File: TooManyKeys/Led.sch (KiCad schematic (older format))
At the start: 2 parts

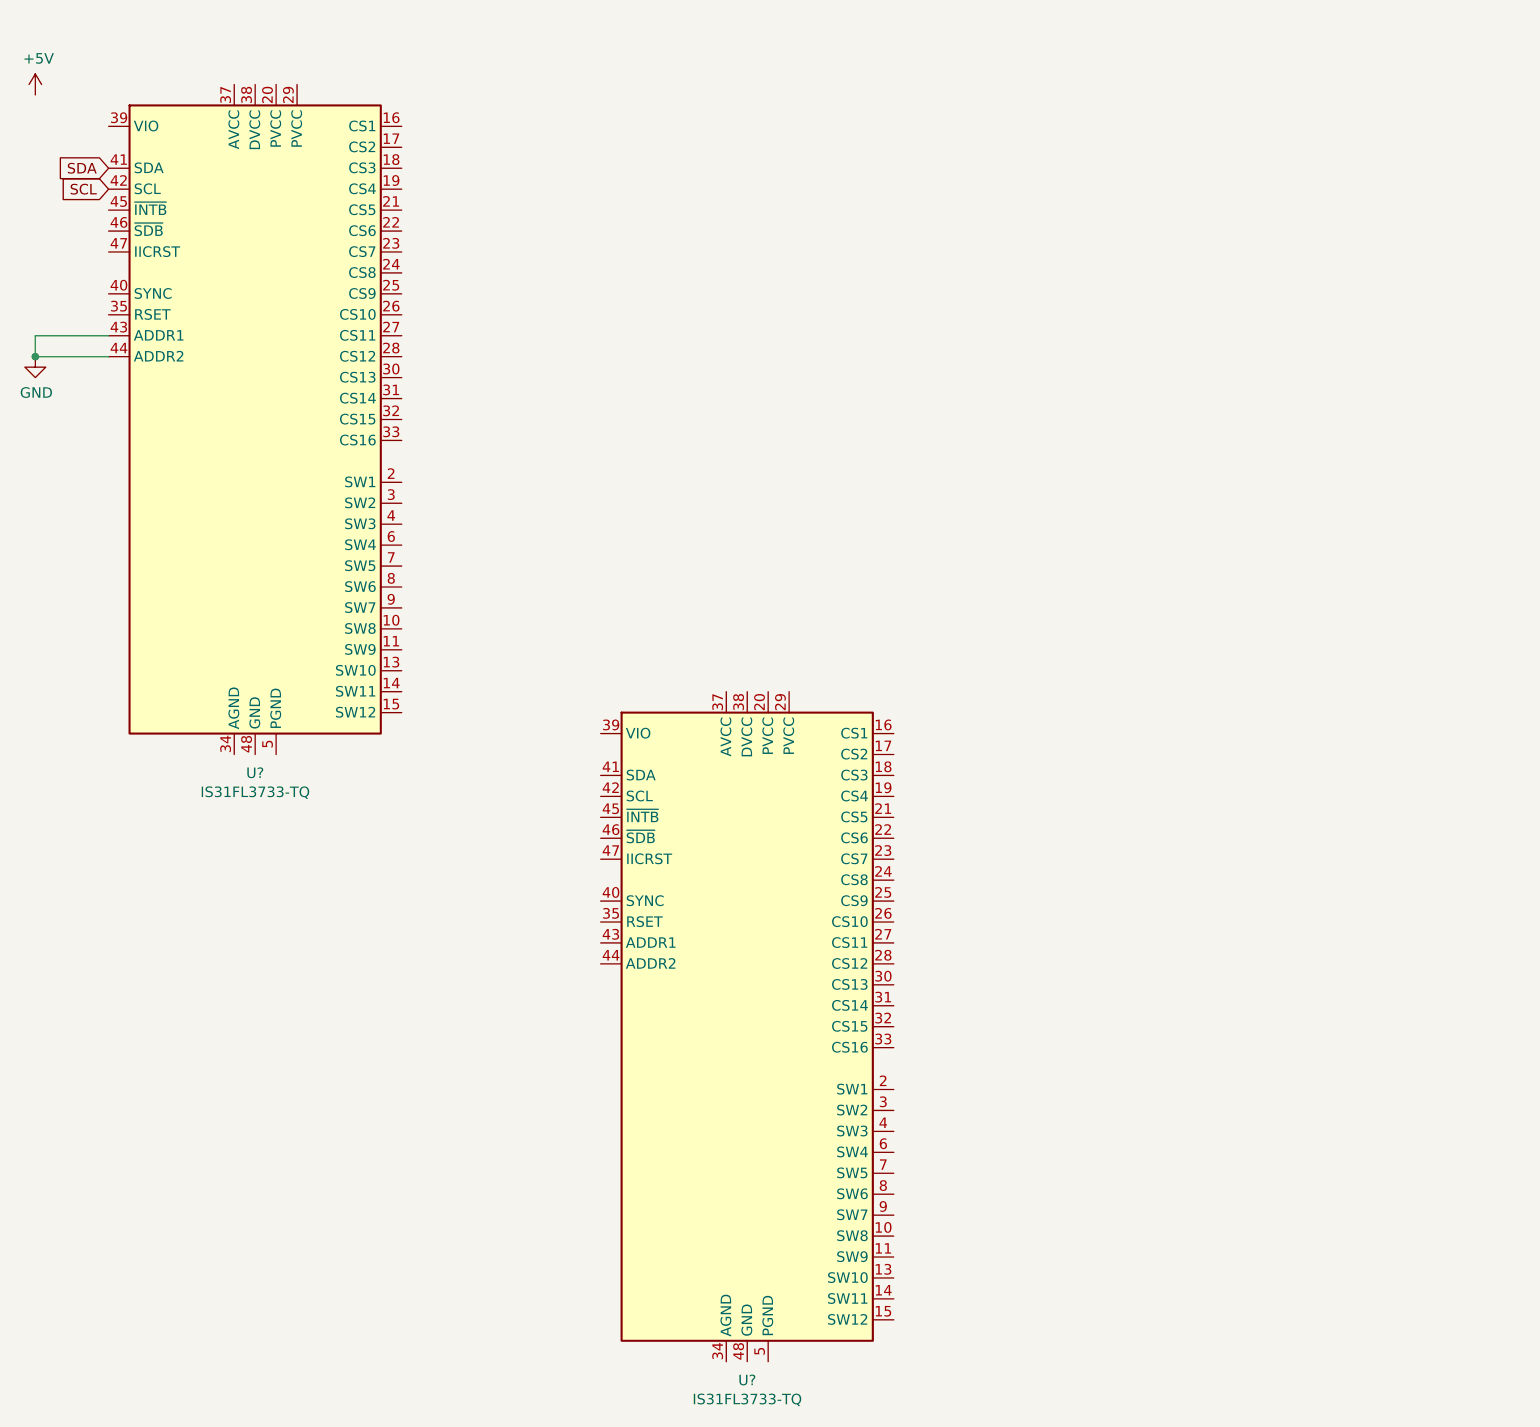
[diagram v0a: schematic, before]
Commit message: led work
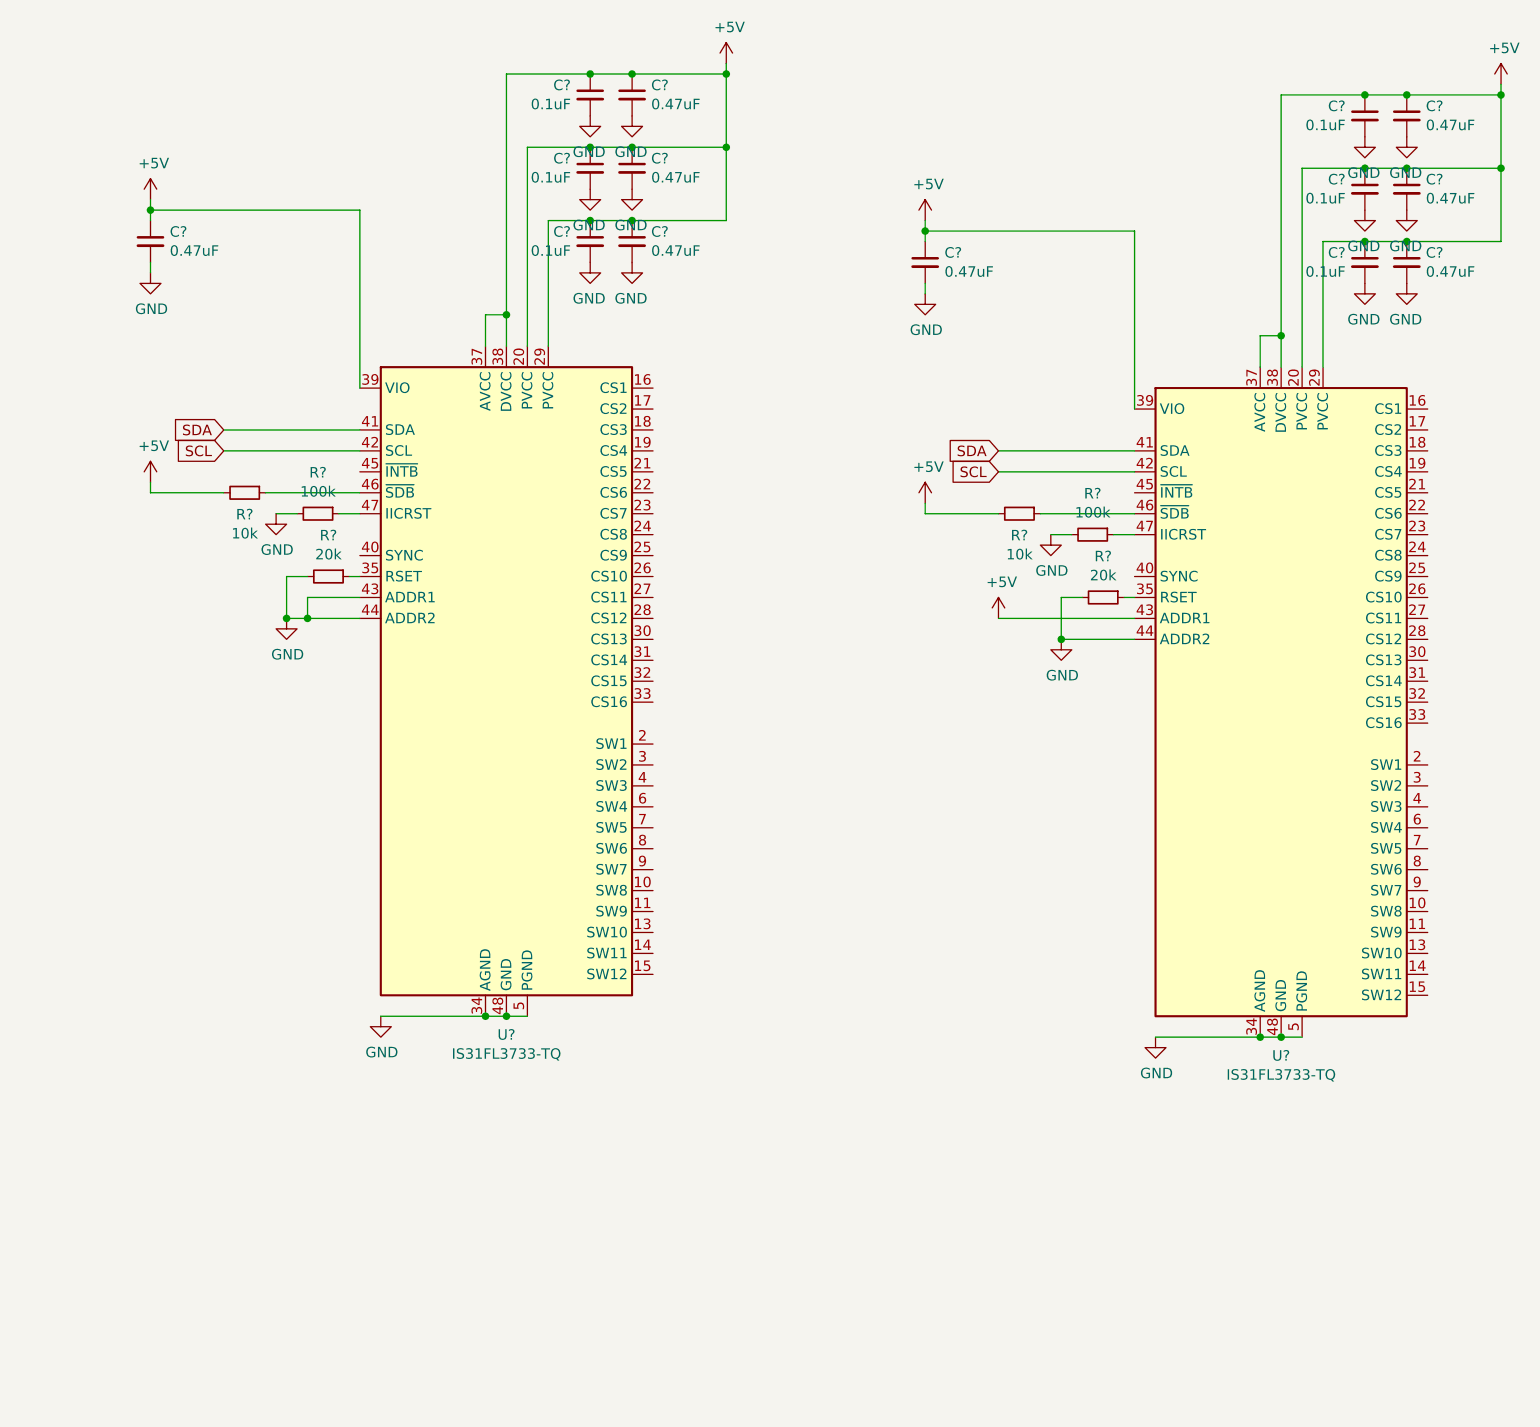
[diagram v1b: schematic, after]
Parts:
- removed U?: IS31FL3733-TQ, Package_QFP:TQFP-48-1EP_7x7mm_P0.5mm_EP5x5mm, symbol Driver_LED:IS31FL3733-TQ
- added C? (x8): 0.47uF, symbol Device:C_Small
- added C? (x6): 0.1uF, symbol Device:C_Small
- added R? (x2): 100k, symbol Device:R_Small
- added R? (x2): 20k, symbol Device:R_Small
- added R? (x2): 10k, symbol Device:R_Small
- added U?: IS31FL3733-TQ, Package_QFP:TQFP-48-1EP_7x7mm_P0.5mm_EP5x5mm, symbol Driver_LED:IS31FL3733-TQ
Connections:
- net +5V: now also U?.20 (PVCC), U?.29 (PVCC), U?.37 (AVCC), U?.38 (DVCC), U?.39 (VIO), C?.1, C?.1, C?.1, C?.1, C?.1, C?.1, C?.1, C?.1, C?.1, C?.1, C?.1, C?.1, C?.1, C?.1, R?.2, R?.2, U?.20 (PVCC), U?.29 (PVCC), U?.37 (AVCC), U?.38 (DVCC), U?.39 (VIO), U?.43 (ADDR1)
- net GND: now also U?.12 (PGND), U?.34 (AGND), U?.48 (GND), U?.49 (GND), U?.5 (PGND), C?.2, C?.2, C?.2, C?.2, C?.2, C?.2, C?.2, C?.2, C?.2, C?.2, C?.2, C?.2, C?.2, C?.2, R?.2, R?.2, R?.2, R?.2, U?.12 (PGND), U?.34 (AGND), U?.44 (ADDR2), U?.48 (GND), U?.49 (GND), U?.5 (PGND)
- net SCL: now also U?.42 (SCL)
- net SDA: now also U?.41 (SDA)
- net at U?.35 (RSET): now also R?.1
- net at U?.46 (~SDB): now also R?.1
- net at U?.47 (IICRST): now also R?.1
- new net: R?.1, U?.35 (RSET)
- new net: R?.1, U?.46 (~SDB)
- new net: R?.1, U?.47 (IICRST)
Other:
- moved on the sheet: U?

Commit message: Adding led matrix
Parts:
- added LED? (x64): XZMDKCBDDG45S-9, XZMDKCBDDG45S9, symbol SamacSys_Parts:XZMDKCBDDG45S-9
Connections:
- new net CS1: LED?.2 (COMMON_ANODE), LED?.2 (COMMON_ANODE), LED?.2 (COMMON_ANODE), LED?.2 (COMMON_ANODE)
- new net CS10: LED?.2 (COMMON_ANODE), LED?.2 (COMMON_ANODE), LED?.2 (COMMON_ANODE), LED?.2 (COMMON_ANODE)
- new net CS11: LED?.2 (COMMON_ANODE), LED?.2 (COMMON_ANODE), LED?.2 (COMMON_ANODE), LED?.2 (COMMON_ANODE)
- new net CS12: LED?.2 (COMMON_ANODE), LED?.2 (COMMON_ANODE), LED?.2 (COMMON_ANODE), LED?.2 (COMMON_ANODE)
- new net CS13: LED?.2 (COMMON_ANODE), LED?.2 (COMMON_ANODE), LED?.2 (COMMON_ANODE), LED?.2 (COMMON_ANODE)
- new net CS14: LED?.2 (COMMON_ANODE), LED?.2 (COMMON_ANODE), LED?.2 (COMMON_ANODE), LED?.2 (COMMON_ANODE)
- new net CS15: LED?.2 (COMMON_ANODE), LED?.2 (COMMON_ANODE), LED?.2 (COMMON_ANODE), LED?.2 (COMMON_ANODE)
- new net CS16: LED?.2 (COMMON_ANODE), LED?.2 (COMMON_ANODE), LED?.2 (COMMON_ANODE), LED?.2 (COMMON_ANODE)
- new net CS2: LED?.2 (COMMON_ANODE), LED?.2 (COMMON_ANODE), LED?.2 (COMMON_ANODE), LED?.2 (COMMON_ANODE)
- new net CS3: LED?.2 (COMMON_ANODE), LED?.2 (COMMON_ANODE), LED?.2 (COMMON_ANODE), LED?.2 (COMMON_ANODE)
- new net CS4: LED?.2 (COMMON_ANODE), LED?.2 (COMMON_ANODE), LED?.2 (COMMON_ANODE), LED?.2 (COMMON_ANODE)
- new net CS5: LED?.2 (COMMON_ANODE), LED?.2 (COMMON_ANODE), LED?.2 (COMMON_ANODE), LED?.2 (COMMON_ANODE)
- new net CS6: LED?.2 (COMMON_ANODE), LED?.2 (COMMON_ANODE), LED?.2 (COMMON_ANODE), LED?.2 (COMMON_ANODE)
- new net CS7: LED?.2 (COMMON_ANODE), LED?.2 (COMMON_ANODE), LED?.2 (COMMON_ANODE), LED?.2 (COMMON_ANODE)
- new net CS8: LED?.2 (COMMON_ANODE), LED?.2 (COMMON_ANODE), LED?.2 (COMMON_ANODE), LED?.2 (COMMON_ANODE)
- new net CS9: LED?.2 (COMMON_ANODE), LED?.2 (COMMON_ANODE), LED?.2 (COMMON_ANODE), LED?.2 (COMMON_ANODE)
- new net SW1: LED?.4 (CATHODE_GREEN), LED?.4 (CATHODE_GREEN), LED?.4 (CATHODE_GREEN), LED?.4 (CATHODE_GREEN), LED?.4 (CATHODE_GREEN), LED?.4 (CATHODE_GREEN), LED?.4 (CATHODE_GREEN), LED?.4 (CATHODE_GREEN), LED?.4 (CATHODE_GREEN), LED?.4 (CATHODE_GREEN), LED?.4 (CATHODE_GREEN), LED?.4 (CATHODE_GREEN), LED?.4 (CATHODE_GREEN), LED?.4 (CATHODE_GREEN), LED?.4 (CATHODE_GREEN), LED?.4 (CATHODE_GREEN)
- new net SW10: LED?.4 (CATHODE_GREEN), LED?.4 (CATHODE_GREEN), LED?.4 (CATHODE_GREEN), LED?.4 (CATHODE_GREEN), LED?.4 (CATHODE_GREEN), LED?.4 (CATHODE_GREEN), LED?.4 (CATHODE_GREEN), LED?.4 (CATHODE_GREEN), LED?.4 (CATHODE_GREEN), LED?.4 (CATHODE_GREEN), LED?.4 (CATHODE_GREEN), LED?.4 (CATHODE_GREEN), LED?.4 (CATHODE_GREEN), LED?.4 (CATHODE_GREEN), LED?.4 (CATHODE_GREEN), LED?.4 (CATHODE_GREEN)
- new net SW11: LED?.1 (CATHODE_RED), LED?.1 (CATHODE_RED), LED?.1 (CATHODE_RED), LED?.1 (CATHODE_RED), LED?.1 (CATHODE_RED), LED?.1 (CATHODE_RED), LED?.1 (CATHODE_RED), LED?.1 (CATHODE_RED), LED?.1 (CATHODE_RED), LED?.1 (CATHODE_RED), LED?.1 (CATHODE_RED), LED?.1 (CATHODE_RED), LED?.1 (CATHODE_RED), LED?.1 (CATHODE_RED), LED?.1 (CATHODE_RED), LED?.1 (CATHODE_RED)
- new net SW12: LED?.3 (CATHODE_BLUE), LED?.3 (CATHODE_BLUE), LED?.3 (CATHODE_BLUE), LED?.3 (CATHODE_BLUE), LED?.3 (CATHODE_BLUE), LED?.3 (CATHODE_BLUE), LED?.3 (CATHODE_BLUE), LED?.3 (CATHODE_BLUE), LED?.3 (CATHODE_BLUE), LED?.3 (CATHODE_BLUE), LED?.3 (CATHODE_BLUE), LED?.3 (CATHODE_BLUE), LED?.3 (CATHODE_BLUE), LED?.3 (CATHODE_BLUE), LED?.3 (CATHODE_BLUE), LED?.3 (CATHODE_BLUE)
- new net SW2: LED?.1 (CATHODE_RED), LED?.1 (CATHODE_RED), LED?.1 (CATHODE_RED), LED?.1 (CATHODE_RED), LED?.1 (CATHODE_RED), LED?.1 (CATHODE_RED), LED?.1 (CATHODE_RED), LED?.1 (CATHODE_RED), LED?.1 (CATHODE_RED), LED?.1 (CATHODE_RED), LED?.1 (CATHODE_RED), LED?.1 (CATHODE_RED), LED?.1 (CATHODE_RED), LED?.1 (CATHODE_RED), LED?.1 (CATHODE_RED), LED?.1 (CATHODE_RED)
- new net SW3: LED?.3 (CATHODE_BLUE), LED?.3 (CATHODE_BLUE), LED?.3 (CATHODE_BLUE), LED?.3 (CATHODE_BLUE), LED?.3 (CATHODE_BLUE), LED?.3 (CATHODE_BLUE), LED?.3 (CATHODE_BLUE), LED?.3 (CATHODE_BLUE), LED?.3 (CATHODE_BLUE), LED?.3 (CATHODE_BLUE), LED?.3 (CATHODE_BLUE), LED?.3 (CATHODE_BLUE), LED?.3 (CATHODE_BLUE), LED?.3 (CATHODE_BLUE), LED?.3 (CATHODE_BLUE), LED?.3 (CATHODE_BLUE)
- new net SW4: LED?.4 (CATHODE_GREEN), LED?.4 (CATHODE_GREEN), LED?.4 (CATHODE_GREEN), LED?.4 (CATHODE_GREEN), LED?.4 (CATHODE_GREEN), LED?.4 (CATHODE_GREEN), LED?.4 (CATHODE_GREEN), LED?.4 (CATHODE_GREEN), LED?.4 (CATHODE_GREEN), LED?.4 (CATHODE_GREEN), LED?.4 (CATHODE_GREEN), LED?.4 (CATHODE_GREEN), LED?.4 (CATHODE_GREEN), LED?.4 (CATHODE_GREEN), LED?.4 (CATHODE_GREEN), LED?.4 (CATHODE_GREEN)
- new net SW5: LED?.1 (CATHODE_RED), LED?.1 (CATHODE_RED), LED?.1 (CATHODE_RED), LED?.1 (CATHODE_RED), LED?.1 (CATHODE_RED), LED?.1 (CATHODE_RED), LED?.1 (CATHODE_RED), LED?.1 (CATHODE_RED), LED?.1 (CATHODE_RED), LED?.1 (CATHODE_RED), LED?.1 (CATHODE_RED), LED?.1 (CATHODE_RED), LED?.1 (CATHODE_RED), LED?.1 (CATHODE_RED), LED?.1 (CATHODE_RED), LED?.1 (CATHODE_RED)
- new net SW6: LED?.3 (CATHODE_BLUE), LED?.3 (CATHODE_BLUE), LED?.3 (CATHODE_BLUE), LED?.3 (CATHODE_BLUE), LED?.3 (CATHODE_BLUE), LED?.3 (CATHODE_BLUE), LED?.3 (CATHODE_BLUE), LED?.3 (CATHODE_BLUE), LED?.3 (CATHODE_BLUE), LED?.3 (CATHODE_BLUE), LED?.3 (CATHODE_BLUE), LED?.3 (CATHODE_BLUE), LED?.3 (CATHODE_BLUE), LED?.3 (CATHODE_BLUE), LED?.3 (CATHODE_BLUE), LED?.3 (CATHODE_BLUE)
- new net SW7: LED?.4 (CATHODE_GREEN), LED?.4 (CATHODE_GREEN), LED?.4 (CATHODE_GREEN), LED?.4 (CATHODE_GREEN), LED?.4 (CATHODE_GREEN), LED?.4 (CATHODE_GREEN), LED?.4 (CATHODE_GREEN), LED?.4 (CATHODE_GREEN), LED?.4 (CATHODE_GREEN), LED?.4 (CATHODE_GREEN), LED?.4 (CATHODE_GREEN), LED?.4 (CATHODE_GREEN), LED?.4 (CATHODE_GREEN), LED?.4 (CATHODE_GREEN), LED?.4 (CATHODE_GREEN), LED?.4 (CATHODE_GREEN)
- new net SW8: LED?.1 (CATHODE_RED), LED?.1 (CATHODE_RED), LED?.1 (CATHODE_RED), LED?.1 (CATHODE_RED), LED?.1 (CATHODE_RED), LED?.1 (CATHODE_RED), LED?.1 (CATHODE_RED), LED?.1 (CATHODE_RED), LED?.1 (CATHODE_RED), LED?.1 (CATHODE_RED), LED?.1 (CATHODE_RED), LED?.1 (CATHODE_RED), LED?.1 (CATHODE_RED), LED?.1 (CATHODE_RED), LED?.1 (CATHODE_RED), LED?.1 (CATHODE_RED)
- new net SW9: LED?.3 (CATHODE_BLUE), LED?.3 (CATHODE_BLUE), LED?.3 (CATHODE_BLUE), LED?.3 (CATHODE_BLUE), LED?.3 (CATHODE_BLUE), LED?.3 (CATHODE_BLUE), LED?.3 (CATHODE_BLUE), LED?.3 (CATHODE_BLUE), LED?.3 (CATHODE_BLUE), LED?.3 (CATHODE_BLUE), LED?.3 (CATHODE_BLUE), LED?.3 (CATHODE_BLUE), LED?.3 (CATHODE_BLUE), LED?.3 (CATHODE_BLUE), LED?.3 (CATHODE_BLUE), LED?.3 (CATHODE_BLUE)
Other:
- moved on the sheet: C?, R?, U?

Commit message: V1 Schematics
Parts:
- removed C? (x8): 0.47uF, symbol Device:C_Small
- removed C? (x6): 0.1uF, symbol Device:C_Small
- removed R? (x2): 100k, symbol Device:R_Small
- removed R? (x2): 20k, symbol Device:R_Small
- removed R? (x2): 10k, symbol Device:R_Small
- removed U? (x2): IS31FL3733-TQ, Package_QFP:TQFP-48-1EP_7x7mm_P0.5mm_EP5x5mm, symbol Driver_LED:IS31FL3733-TQ
- added LED? (x47): XZMDKCBDDG45S-9, XZMDKCBDDG45S9, symbol SamacSys_Parts:XZMDKCBDDG45S-9
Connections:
- new net CS17: LED?.2 (COMMON_ANODE), LED?.2 (COMMON_ANODE), LED?.2 (COMMON_ANODE), LED?.2 (COMMON_ANODE)
- new net CS18: LED?.2 (COMMON_ANODE), LED?.2 (COMMON_ANODE), LED?.2 (COMMON_ANODE), LED?.2 (COMMON_ANODE)
- new net CS19: LED?.2 (COMMON_ANODE), LED?.2 (COMMON_ANODE), LED?.2 (COMMON_ANODE), LED?.2 (COMMON_ANODE)
- new net CS20: LED?.2 (COMMON_ANODE), LED?.2 (COMMON_ANODE), LED?.2 (COMMON_ANODE), LED?.2 (COMMON_ANODE)
- new net CS21: LED?.2 (COMMON_ANODE), LED?.2 (COMMON_ANODE), LED?.2 (COMMON_ANODE), LED?.2 (COMMON_ANODE)
- new net CS22: LED?.2 (COMMON_ANODE), LED?.2 (COMMON_ANODE), LED?.2 (COMMON_ANODE), LED?.2 (COMMON_ANODE)
- new net CS23: LED?.2 (COMMON_ANODE), LED?.2 (COMMON_ANODE), LED?.2 (COMMON_ANODE), LED?.2 (COMMON_ANODE)
- new net CS24: LED?.2 (COMMON_ANODE), LED?.2 (COMMON_ANODE), LED?.2 (COMMON_ANODE), LED?.2 (COMMON_ANODE)
- new net CS25: LED?.2 (COMMON_ANODE), LED?.2 (COMMON_ANODE), LED?.2 (COMMON_ANODE), LED?.2 (COMMON_ANODE)
- new net CS26: LED?.2 (COMMON_ANODE), LED?.2 (COMMON_ANODE), LED?.2 (COMMON_ANODE), LED?.2 (COMMON_ANODE)
- new net CS27: LED?.2 (COMMON_ANODE), LED?.2 (COMMON_ANODE), LED?.2 (COMMON_ANODE), LED?.2 (COMMON_ANODE)
- new net CS28: LED?.2 (COMMON_ANODE), LED?.2 (COMMON_ANODE), LED?.2 (COMMON_ANODE)
- new net SW13: LED?.4 (CATHODE_GREEN), LED?.4 (CATHODE_GREEN), LED?.4 (CATHODE_GREEN), LED?.4 (CATHODE_GREEN), LED?.4 (CATHODE_GREEN), LED?.4 (CATHODE_GREEN), LED?.4 (CATHODE_GREEN), LED?.4 (CATHODE_GREEN), LED?.4 (CATHODE_GREEN), LED?.4 (CATHODE_GREEN), LED?.4 (CATHODE_GREEN), LED?.4 (CATHODE_GREEN)
- new net SW14: LED?.1 (CATHODE_RED), LED?.1 (CATHODE_RED), LED?.1 (CATHODE_RED), LED?.1 (CATHODE_RED), LED?.1 (CATHODE_RED), LED?.1 (CATHODE_RED), LED?.1 (CATHODE_RED), LED?.1 (CATHODE_RED), LED?.1 (CATHODE_RED), LED?.1 (CATHODE_RED), LED?.1 (CATHODE_RED), LED?.1 (CATHODE_RED)
- new net SW15: LED?.3 (CATHODE_BLUE), LED?.3 (CATHODE_BLUE), LED?.3 (CATHODE_BLUE), LED?.3 (CATHODE_BLUE), LED?.3 (CATHODE_BLUE), LED?.3 (CATHODE_BLUE), LED?.3 (CATHODE_BLUE), LED?.3 (CATHODE_BLUE), LED?.3 (CATHODE_BLUE), LED?.3 (CATHODE_BLUE), LED?.3 (CATHODE_BLUE), LED?.3 (CATHODE_BLUE)
- new net SW16: LED?.4 (CATHODE_GREEN), LED?.4 (CATHODE_GREEN), LED?.4 (CATHODE_GREEN), LED?.4 (CATHODE_GREEN), LED?.4 (CATHODE_GREEN), LED?.4 (CATHODE_GREEN), LED?.4 (CATHODE_GREEN), LED?.4 (CATHODE_GREEN), LED?.4 (CATHODE_GREEN), LED?.4 (CATHODE_GREEN), LED?.4 (CATHODE_GREEN), LED?.4 (CATHODE_GREEN)
- new net SW17: LED?.1 (CATHODE_RED), LED?.1 (CATHODE_RED), LED?.1 (CATHODE_RED), LED?.1 (CATHODE_RED), LED?.1 (CATHODE_RED), LED?.1 (CATHODE_RED), LED?.1 (CATHODE_RED), LED?.1 (CATHODE_RED), LED?.1 (CATHODE_RED), LED?.1 (CATHODE_RED), LED?.1 (CATHODE_RED), LED?.1 (CATHODE_RED)
- new net SW18: LED?.3 (CATHODE_BLUE), LED?.3 (CATHODE_BLUE), LED?.3 (CATHODE_BLUE), LED?.3 (CATHODE_BLUE), LED?.3 (CATHODE_BLUE), LED?.3 (CATHODE_BLUE), LED?.3 (CATHODE_BLUE), LED?.3 (CATHODE_BLUE), LED?.3 (CATHODE_BLUE), LED?.3 (CATHODE_BLUE), LED?.3 (CATHODE_BLUE), LED?.3 (CATHODE_BLUE)
- new net SW19: LED?.4 (CATHODE_GREEN), LED?.4 (CATHODE_GREEN), LED?.4 (CATHODE_GREEN), LED?.4 (CATHODE_GREEN), LED?.4 (CATHODE_GREEN), LED?.4 (CATHODE_GREEN), LED?.4 (CATHODE_GREEN), LED?.4 (CATHODE_GREEN), LED?.4 (CATHODE_GREEN), LED?.4 (CATHODE_GREEN), LED?.4 (CATHODE_GREEN), LED?.4 (CATHODE_GREEN)
- new net SW20: LED?.1 (CATHODE_RED), LED?.1 (CATHODE_RED), LED?.1 (CATHODE_RED), LED?.1 (CATHODE_RED), LED?.1 (CATHODE_RED), LED?.1 (CATHODE_RED), LED?.1 (CATHODE_RED), LED?.1 (CATHODE_RED), LED?.1 (CATHODE_RED), LED?.1 (CATHODE_RED), LED?.1 (CATHODE_RED), LED?.1 (CATHODE_RED)
- new net SW21: LED?.3 (CATHODE_BLUE), LED?.3 (CATHODE_BLUE), LED?.3 (CATHODE_BLUE), LED?.3 (CATHODE_BLUE), LED?.3 (CATHODE_BLUE), LED?.3 (CATHODE_BLUE), LED?.3 (CATHODE_BLUE), LED?.3 (CATHODE_BLUE), LED?.3 (CATHODE_BLUE), LED?.3 (CATHODE_BLUE), LED?.3 (CATHODE_BLUE), LED?.3 (CATHODE_BLUE)
- new net SW22: LED?.4 (CATHODE_GREEN), LED?.4 (CATHODE_GREEN), LED?.4 (CATHODE_GREEN), LED?.4 (CATHODE_GREEN), LED?.4 (CATHODE_GREEN), LED?.4 (CATHODE_GREEN), LED?.4 (CATHODE_GREEN), LED?.4 (CATHODE_GREEN), LED?.4 (CATHODE_GREEN), LED?.4 (CATHODE_GREEN), LED?.4 (CATHODE_GREEN)
- new net SW23: LED?.1 (CATHODE_RED), LED?.1 (CATHODE_RED), LED?.1 (CATHODE_RED), LED?.1 (CATHODE_RED), LED?.1 (CATHODE_RED), LED?.1 (CATHODE_RED), LED?.1 (CATHODE_RED), LED?.1 (CATHODE_RED), LED?.1 (CATHODE_RED), LED?.1 (CATHODE_RED), LED?.1 (CATHODE_RED)
- new net SW24: LED?.3 (CATHODE_BLUE), LED?.3 (CATHODE_BLUE), LED?.3 (CATHODE_BLUE), LED?.3 (CATHODE_BLUE), LED?.3 (CATHODE_BLUE), LED?.3 (CATHODE_BLUE), LED?.3 (CATHODE_BLUE), LED?.3 (CATHODE_BLUE), LED?.3 (CATHODE_BLUE), LED?.3 (CATHODE_BLUE), LED?.3 (CATHODE_BLUE)
